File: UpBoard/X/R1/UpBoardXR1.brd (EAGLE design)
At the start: 88.9 x 88.6 mm, 75 parts, among them CN1 100nF, CN2 100nF, CN3 100nF, CN4 100nF, IC1 SAM3X8E(ARDUINO), J1 2POSTERMINALBLOCK.25"PITCH, Q6 2N7002E, X1 16POS_RIBBON, X2 16POS_RIBBON, X3 16POS_RIBBON, X4 16POS_RIBBON, Y1 FH1200001, Y2 ABS05

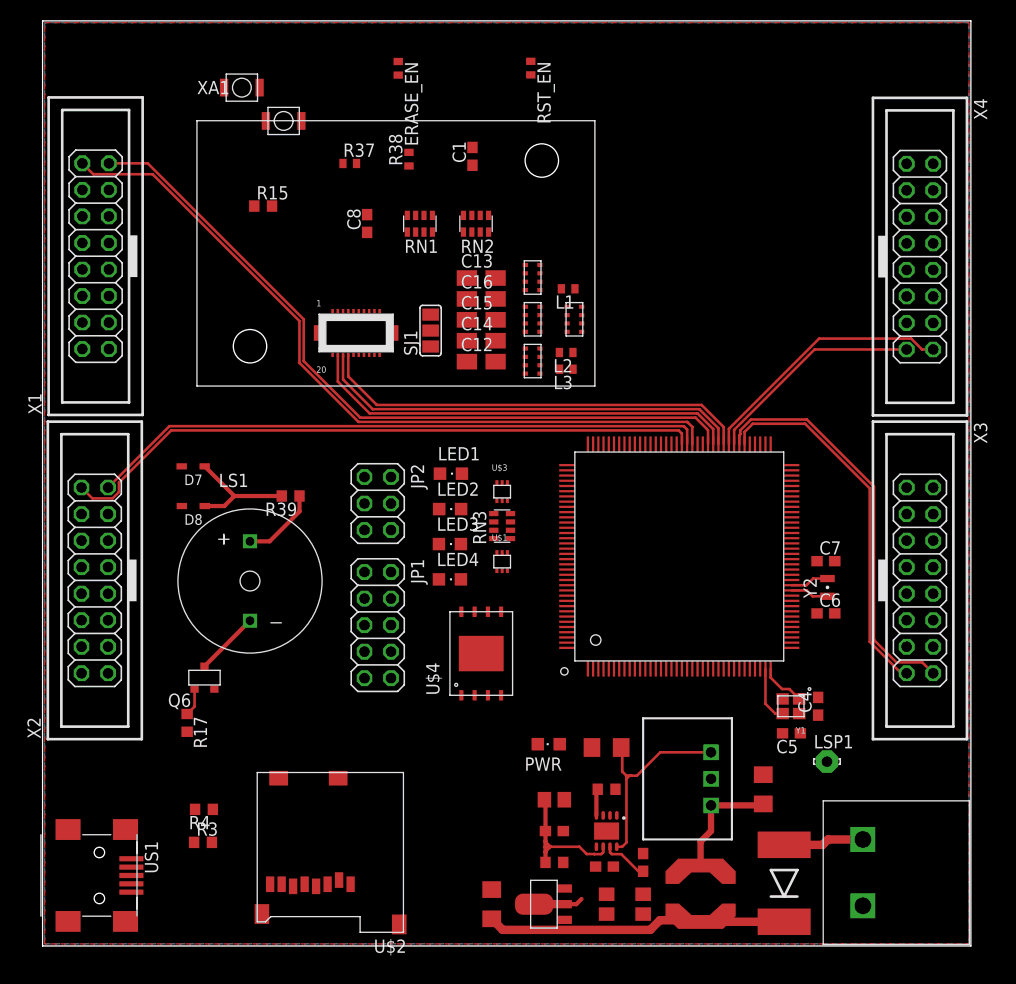
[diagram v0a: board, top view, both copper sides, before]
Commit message: Update R1
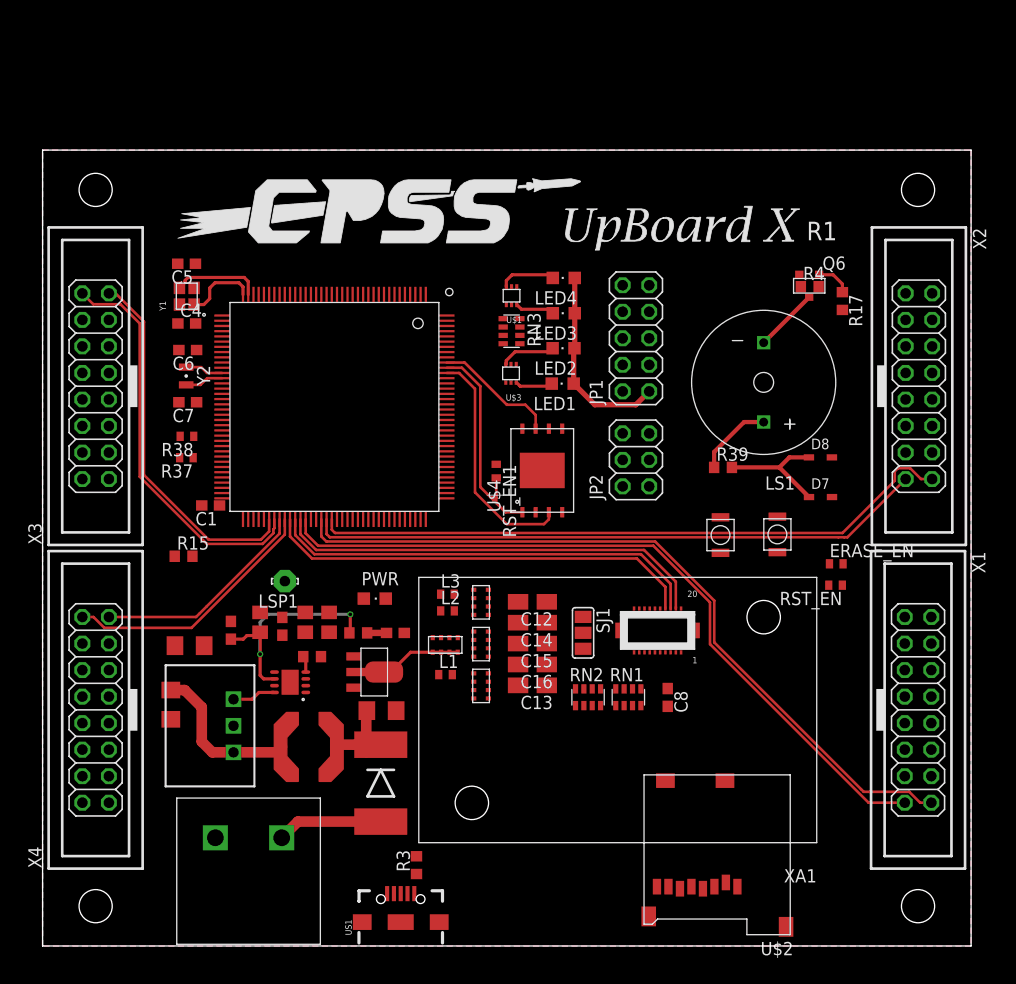
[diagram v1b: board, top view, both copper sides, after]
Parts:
- added RST_EN1: 1K, resistor:R0402
- US1: device adafruit:USB-MINIB -> SparkFun-Connectors:USB-B-MICRO-SMD
- moved X4 90.1 mm to (5.08, 22.6), turned to 90 degrees
- moved X1 89.9 mm to (83.8, 22.6), turned to 270 degrees
- moved X3 81.1 mm to (5.08, 53.6), turned to 90 degrees
- moved X2 81.1 mm to (83.9, 53.6), turned to 270 degrees
- moved R4 76.6 mm to (73.5, 63.1), turned to 0 degrees
- moved R17 74.6 mm to (76.6, 61.7)
- moved C5 73.3 mm to (13.8, 65.3)
- moved C4 70.7 mm to (13.8, 59.6), turned to 0 degrees
- moved Y1 69.9 mm to (13.8, 62.2), turned to 90 degrees
- moved Q6 69.0 mm to (73.4, 63.2), turned to 180 degrees
- moved C6 66.1 mm to (13.9, 57.1), turned to 180 degrees
- moved Y2 64.6 mm to (13.8, 54.6), turned to 270 degrees
- moved ERASE_EN 63.3 mm to (76.0, 36.6), turned to 0 degrees
- moved C7 63.0 mm to (13.9, 52.1), turned to 180 degrees
- moved RESET 62.7 mm to (64.9, 39.3), turned to 0 degrees
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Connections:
- removed net N$13: U$4.P1
- removed net N$14: U$4.P3
- removed net N$15: U$4.P7
- removed net N$3: U$4.P6
- net 3.3V: now also RST_EN1.1, XA1.P$2
- net D6: now also U$4.P7
- net D7: now also RST_EN1.2, U$4.P1
- net D8: now also U$4.P3
- net HV: no longer XA1.P$2, XA1.P$3
- net MISO: no longer U$4.P5
- net MOSI: now also U$4.P5
- net SCK: now also U$4.P6
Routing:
- net 3.3V: track 4.75 -> 29.3 mm
- net D8: track 0.00 -> 22.4 mm
- net D7: track 0.00 -> 22.3 mm
- net HV: track 28.9 -> 9.50 mm
- net PS1-1:BATT_5V: track 19.8 -> 4.19 mm
- net D6: track 0.00 -> 11.9 mm
- net PS1-1:USB_FILTERED: track 13.9 -> 22.7 mm, vias 0 -> 2
- net N$10: track 0.00 -> 5.40 mm
- net N$7: track 0.00 -> 5.32 mm
- net 5V: track 4.46 -> 0.00 mm
- net PS1-1:N$2: track 11.4 -> 15.3 mm
- net N$8: track 0.00 -> 3.79 mm
- net N$38: track 0.00 -> 3.66 mm
- net N$32: track 5.38 -> 8.53 mm
- net N$34: track 4.43 -> 7.05 mm
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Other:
- board size 88.9 x 88.6 mm -> 88.9 x 76.2 mm
- board text added: "R1"
